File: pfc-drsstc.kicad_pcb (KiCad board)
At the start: 2 copper layers, 78.3 x 108.6 mm, 90 parts, among them J1 AC_IN, J2 GDT_PRMY, J3 GDT_SCDY_A, J4 GDT_SCDY_B, J5 12V_IN, J6 PRMY, J7 PHASE_FB, J8 OCP, J9 IF-D95T, Q1 FGA60N65SMD, Q2 FGA60N65SMD, Q3 FGA60N65SMD, Q4 NMOS DPAK, Q5 NMOS DPAK, Q6 PMOS DPAK, Q7 PMOS DPAK, U1 74LS14, U10 INA281A2, U2 74LS74, U3 74LS08, U4 LM311, U5 UCC27423, U6 STM32F103C8Tx, U7 MCP1703Ax-330xxDB, U8 MCP1703Ax-500xxDB, U9 MCP1407, Y1 ATS080B-E

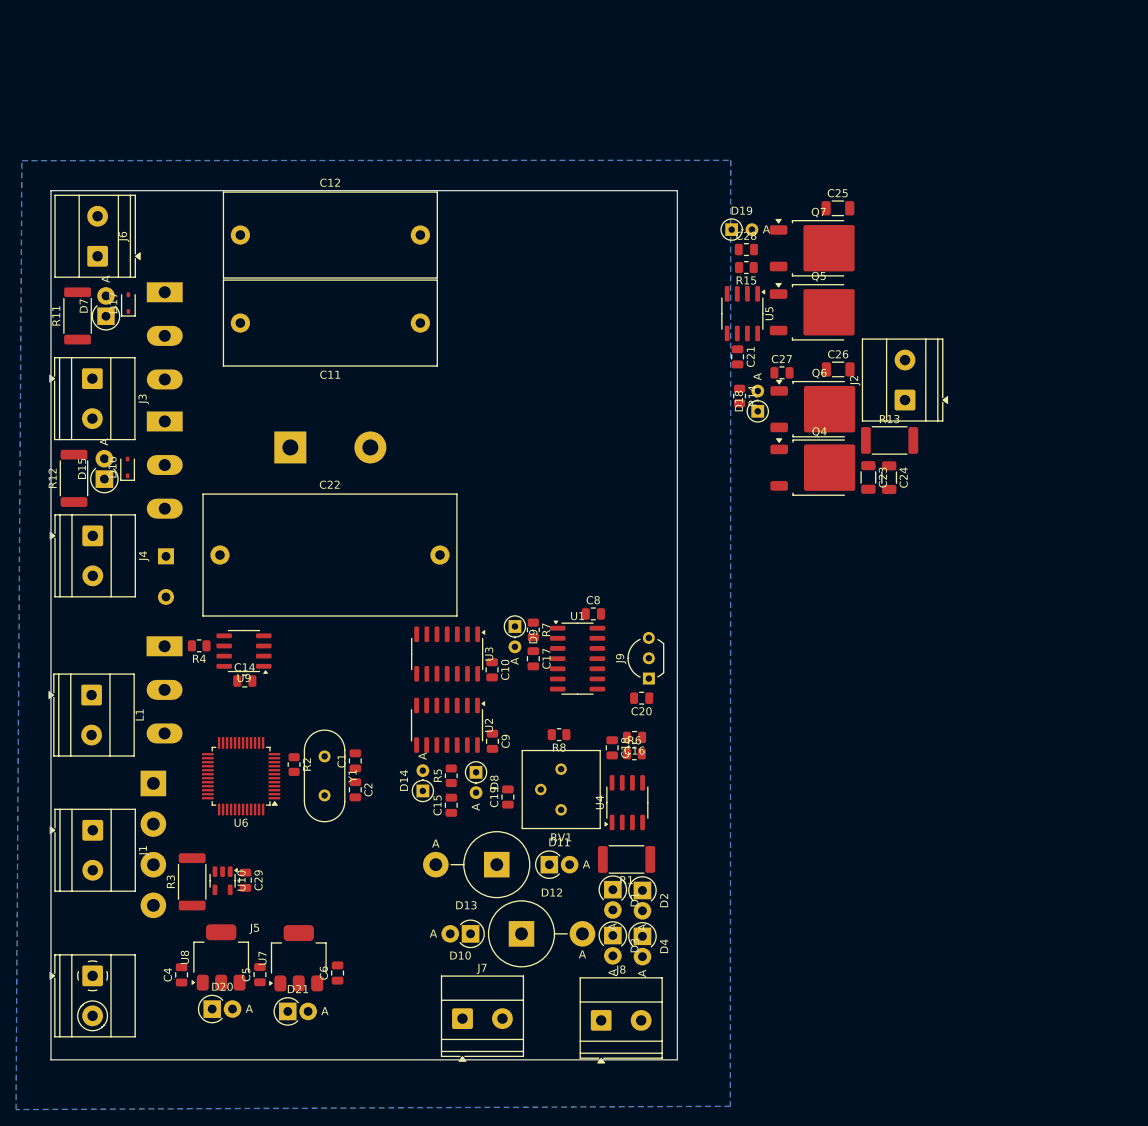
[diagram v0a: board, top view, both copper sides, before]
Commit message: layout nearly complete
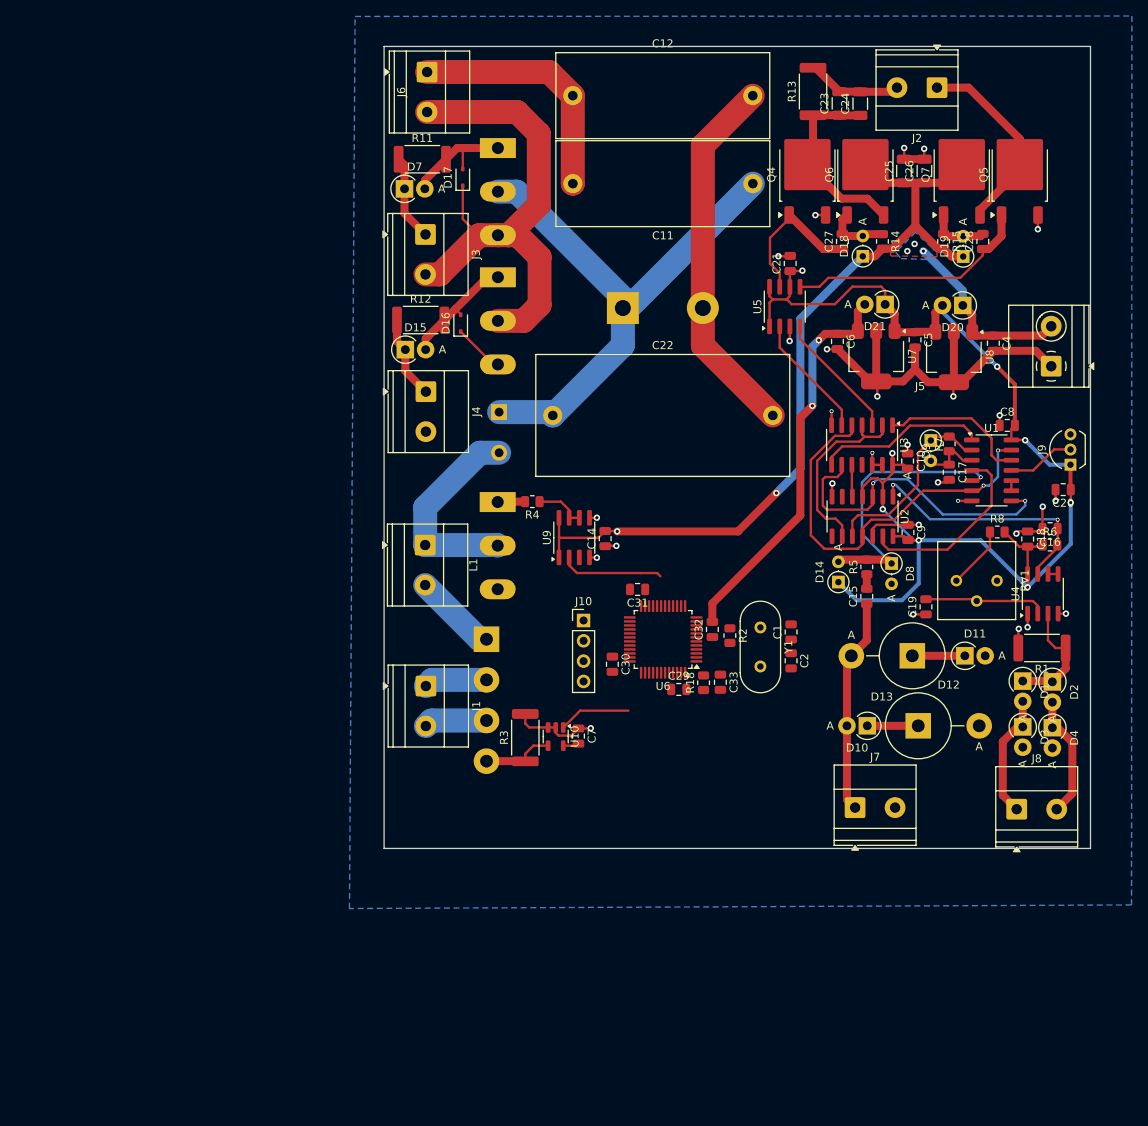
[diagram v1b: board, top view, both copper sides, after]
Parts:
- added C29: 0.1u, Capacitor_SMD:C_0805_2012Metric, F.Cu at (138.7, 119.2)
- added C30: 0.1u, Capacitor_SMD:C_0805_2012Metric, F.Cu at (130.4, 116.0)
- added C31: 0.1u, Capacitor_SMD:C_0805_2012Metric, F.Cu at (133.6, 106.7)
- added C32: 0.1u, Capacitor_SMD:C_0805_2012Metric, F.Cu at (142.9, 111.7)
- added C33: 0.1u, Capacitor_SMD:C_0805_2012Metric, F.Cu at (143.9, 118.2)
- added J10: SWD, Connector_PinHeader_2.54mm:PinHeader_1x04_P2.54mm_Vertical, F.Cu at (126.8, 110.5)
- added R18: 10K, Resistor_SMD:R_0805_2012Metric, F.Cu at (141.8, 118.3)
- moved J5 142.0 mm to (185.3, 78.7), turned to 90 degrees
- moved D20 128.6 mm to (174.2, 71.1), turned to 180 degrees
- moved C4 128.6 mm to (178.0, 75.9), turned to -90 degrees
- moved U8 118.4 mm to (173.1, 77.6), turned to -90 degrees
- moved D21 115.7 mm to (164.5, 71.0), turned to 180 degrees
- moved C5 114.0 mm to (168.2, 75.4), turned to -90 degrees
- moved U7 104.3 mm to (163.4, 77.5), turned to -90 degrees
- moved C6 100.7 mm to (158.5, 75.6), turned to -90 degrees
- moved R8 60.3 mm to (178.5, 99.5), turned to 0 degrees
- moved J9 58.8 mm to (187.7, 91.7)
- moved C20 58.8 mm to (186.8, 94.2)
- moved R1 58.3 mm to (184.1, 114.0)
- moved J8 58.3 mm to (180.9, 134.1)
- moved R6 58.1 mm to (185.1, 101.1)
- moved C16 58.1 mm to (185.1, 99.0)
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- renumbered C29 to C7
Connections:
- J2 pad 1: /DRIVER+ -> /DRIVER-
- J2 pad 2: /DRIVER- -> /DRIVER+
- J6 pad 1: /Power stage/LC_CAPSIDE -> /Power stage/PWR_MIDPT
- J6 pad 2: /Power stage/PWR_MIDPT -> /A-
- U3 pad 1: Net-(U2B-Q) -> Net-(U1-Pad12)
- U3 pad 2: Net-(U2B-C) -> Net-(U2B-Q)
- U3 pad 3: Net-(U5-INA) -> Net-(U5-INB)
- U3 pad 4: Net-(U1-Pad12) -> Net-(U2B-Q)
- U3 pad 5: Net-(U2B-Q) -> Net-(U2B-C)
- U3 pad 6: Net-(U5-INB) -> Net-(U5-INA)
- U6 pad 34: unconnected-(U6-PA13-Pad34) -> /MCU and PFC/SWIO
- U6 pad 37: unconnected-(U6-PA14-Pad37) -> /MCU and PFC/SWCLK
- U6 pad 44: unconnected-(U6-BOOT0-Pad44) -> GND
- U6 pad 7: unconnected-(U6-NRST-Pad7) -> Net-(U6-NRST)
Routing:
- net GND: track 0.00 -> 165.5 mm, vias 0 -> 28
- net +5V: track 0.00 -> 154.9 mm, vias 0 -> 8
- net +12V: track 0.00 -> 126.7 mm, vias 0 -> 5
- net +PWR: track 0.00 -> 69.0 mm
- net /A-: track 0.00 -> 65.8 mm
- net +3.3V: track 0.00 -> 51.8 mm, vias 0 -> 2
- net Net-(U2B-C): track 0.00 -> 50.9 mm, vias 0 -> 2
- net /Feedback controller/INT_SQUARED: track 0.00 -> 40.2 mm, vias 0 -> 2
- net Net-(D14-A): track 0.00 -> 35.6 mm, vias 0 -> 1
- net /Feedback controller/OCP_TRIG: track 0.00 -> 31.7 mm, vias 0 -> 2
- net /Feedback controller/UCC_OUTB: track 0.00 -> 31.2 mm
- net /Power stage/PWR_MIDPT: track 0.00 -> 30.4 mm
- net Net-(D10-A): track 0.00 -> 26.9 mm
- net /MCU and PFC/PFC_SWNODE: track 0.00 -> 25.9 mm
- net /DRIVER-: track 0.00 -> 24.6 mm
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- added copper zone on B.Cu, net +12V
- added copper zone on F.Cu, net +12V
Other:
- board size 78.3 x 108.6 mm -> 88.3 x 100.2 mm
- board text added: "Air flows in from this direction"
